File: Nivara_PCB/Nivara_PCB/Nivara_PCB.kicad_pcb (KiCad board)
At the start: 4 copper layers, 98.8 x 81.2 mm, 160 parts, among them CN1 ANALOG_IN, CN2 RELAY, J1 AUXILIAR, K1 SRA-24VDC-CL, K2 SRA-24VDC-CL, P1 NPN_IN, P2 PNP_IN, P3 D_IN, P4 RUN/STOP, P5 NPN_OUT, P6 PNP_OUT, P7 RS485, P8 ANALOG_OUT., Q1 IRLML0040, Q2 AO3407A, Q3 IRLML0040, Q4 AO3407A, Q5 IRLML6402TRPBF-JSM, SW1 SKRPACE010, SW2 SKRPACE010, U1 2.54-2*2, U10 GP8201S-TC50-EW, U11 LK1802, U12 LTV-357T, U13 LTV-357T, U14 LTV-357T, U15 LTV-357T, U16 LTV-357T, U17 LTV-357T, U18 LTV-357T, U19 GP8303-TC50-EW, U2 FUENTE IN, U3 ESP32-S3-WROOM-1, U4 AP63200WU, U5 RSM3485ECHT_C2992406, U6 LTV-357T, U7 LTV-357T, U8 LTV-357T, U9 LTV-357T

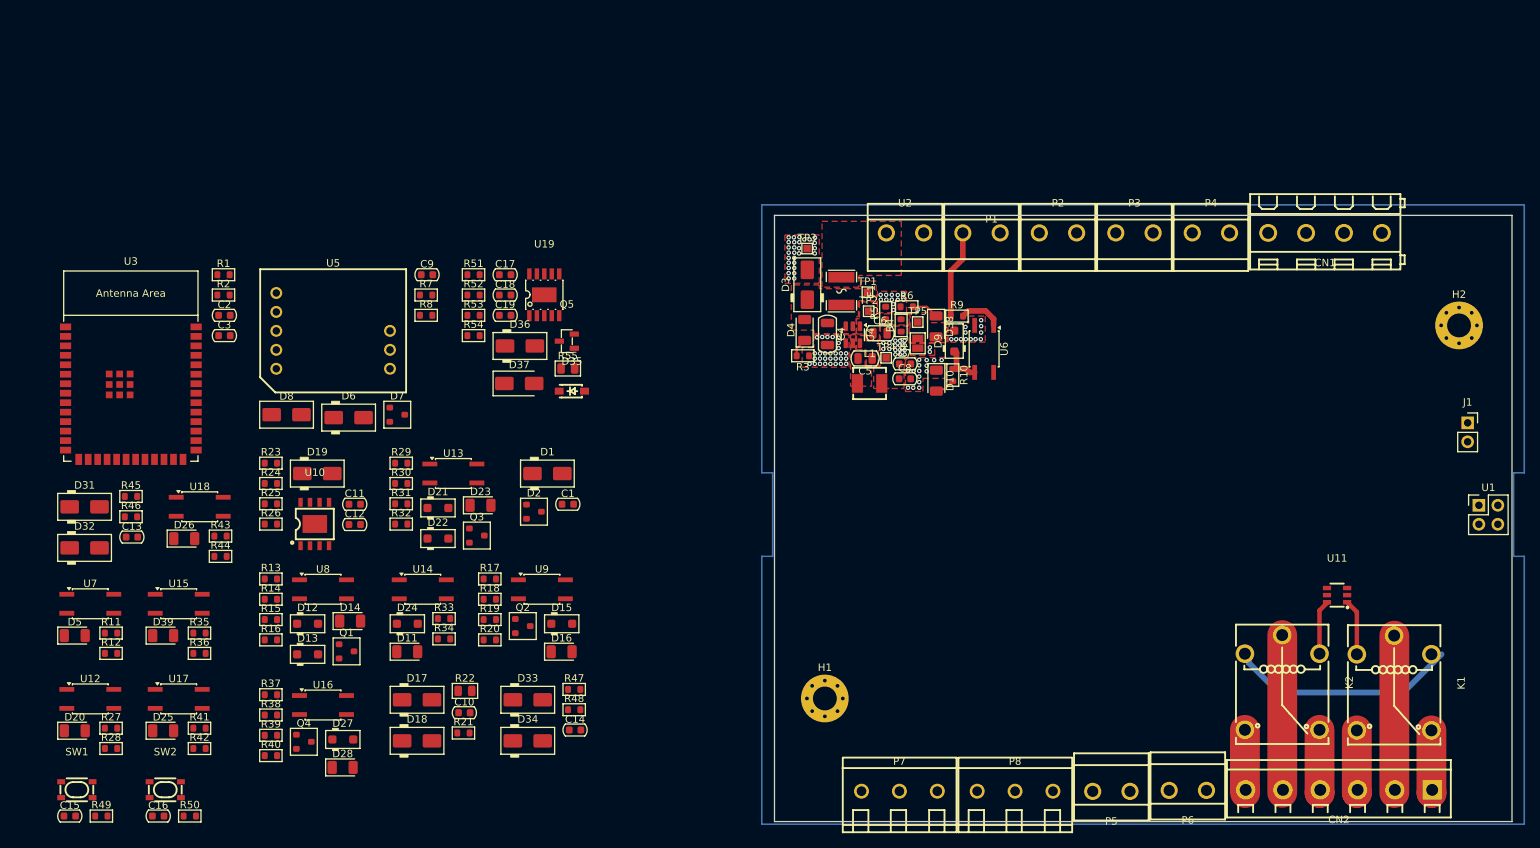
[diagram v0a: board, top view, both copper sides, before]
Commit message: Cambios en el diseño del pcb.
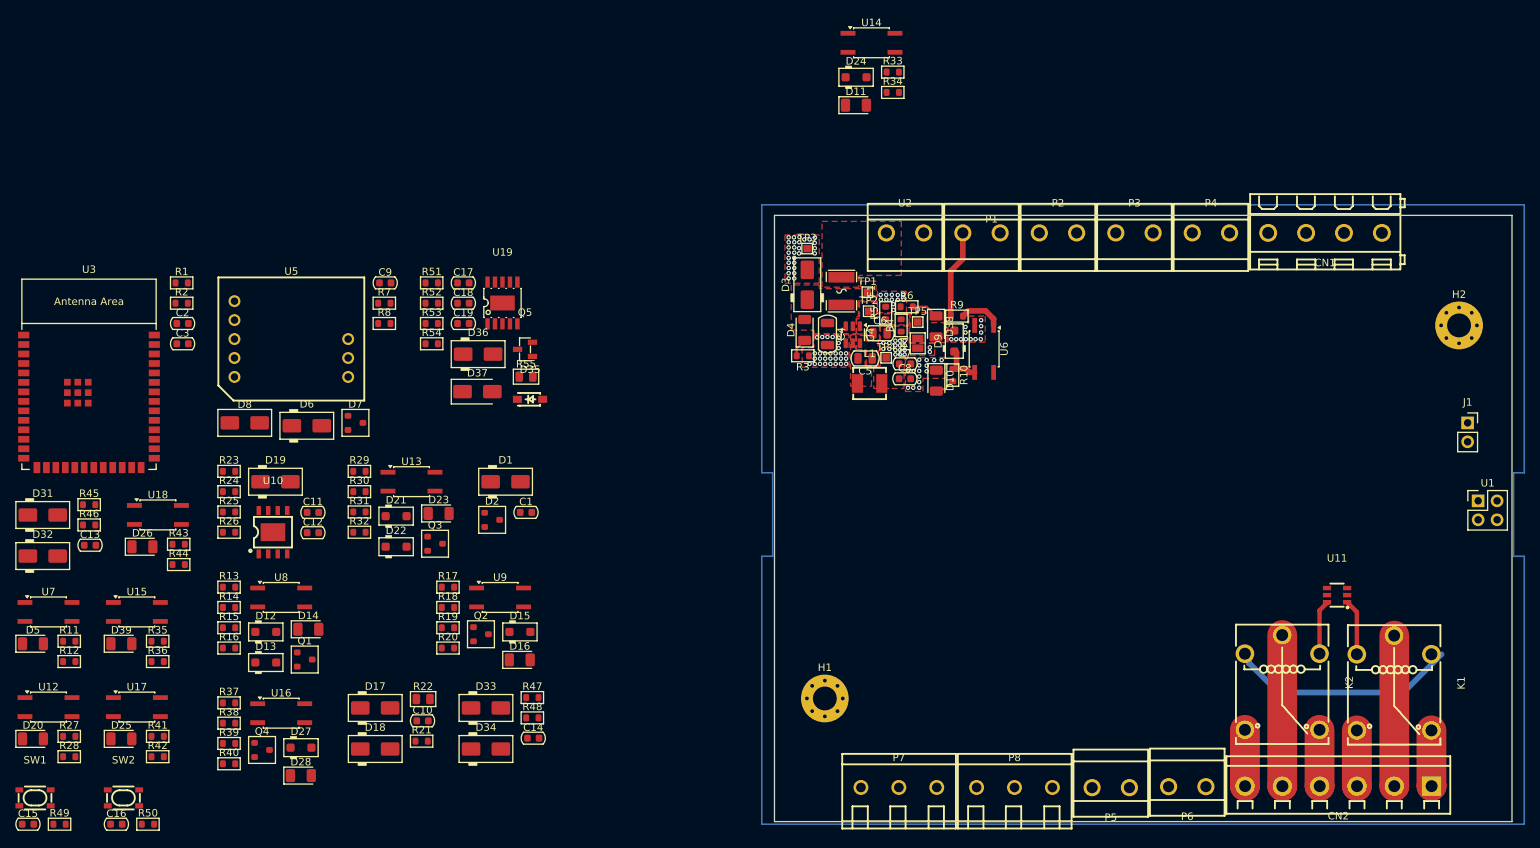
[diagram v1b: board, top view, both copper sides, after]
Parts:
- moved D24 94.8 mm to (178.6, 22.9)
- moved R34 94.8 mm to (183.5, 24.9)
- moved U14 94.8 mm to (180.7, 18.3)
- moved D11 94.8 mm to (178.6, 26.6)
- moved R33 94.8 mm to (183.5, 22.2)
- moved C10 5.71 mm to (120.5, 109.2)
- moved C13 5.71 mm to (75.9, 85.6)
- moved C14 5.71 mm to (135.3, 111.5)
- moved C15 5.71 mm to (67.6, 123.0)
- moved C16 5.71 mm to (79.5, 123.0)
- moved C2 5.71 mm to (88.3, 55.9)
- moved C3 5.71 mm to (88.3, 58.6)
- moved C9 5.71 mm to (115.5, 50.5)
- moved D1 5.71 mm to (131.6, 77.1)
- moved D13 5.71 mm to (99.5, 101.3)
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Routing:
- net /NIVARA_BOARD/RLY_2_NO: track 8.49 -> 7.56 mm
- net /NIVARA_BOARD/RLY_2_NC: track 8.49 -> 7.56 mm
- net /NIVARA_BOARD/RLY_1_NO: track 8.41 -> 7.48 mm
- net /NIVARA_BOARD/RLY_1_NC: track 8.41 -> 7.48 mm
- net /NIVARA_BOARD/RLY_1_C: track 21.1 -> 20.2 mm
- net /NIVARA_BOARD/RLY_2_C: track 21.1 -> 20.3 mm
